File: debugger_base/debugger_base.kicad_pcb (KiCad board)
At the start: 4 copper layers, 58.4 x 38.1 mm, 62 parts, among them SW1 RST_FT, SW2 UART CHx LED enable switch, X1 USB_C_Receptacle_USB2.0_14P, X2 Channel A, X3 Channel B, X4 Channel C, X5 Channel D, Y1 12MHz

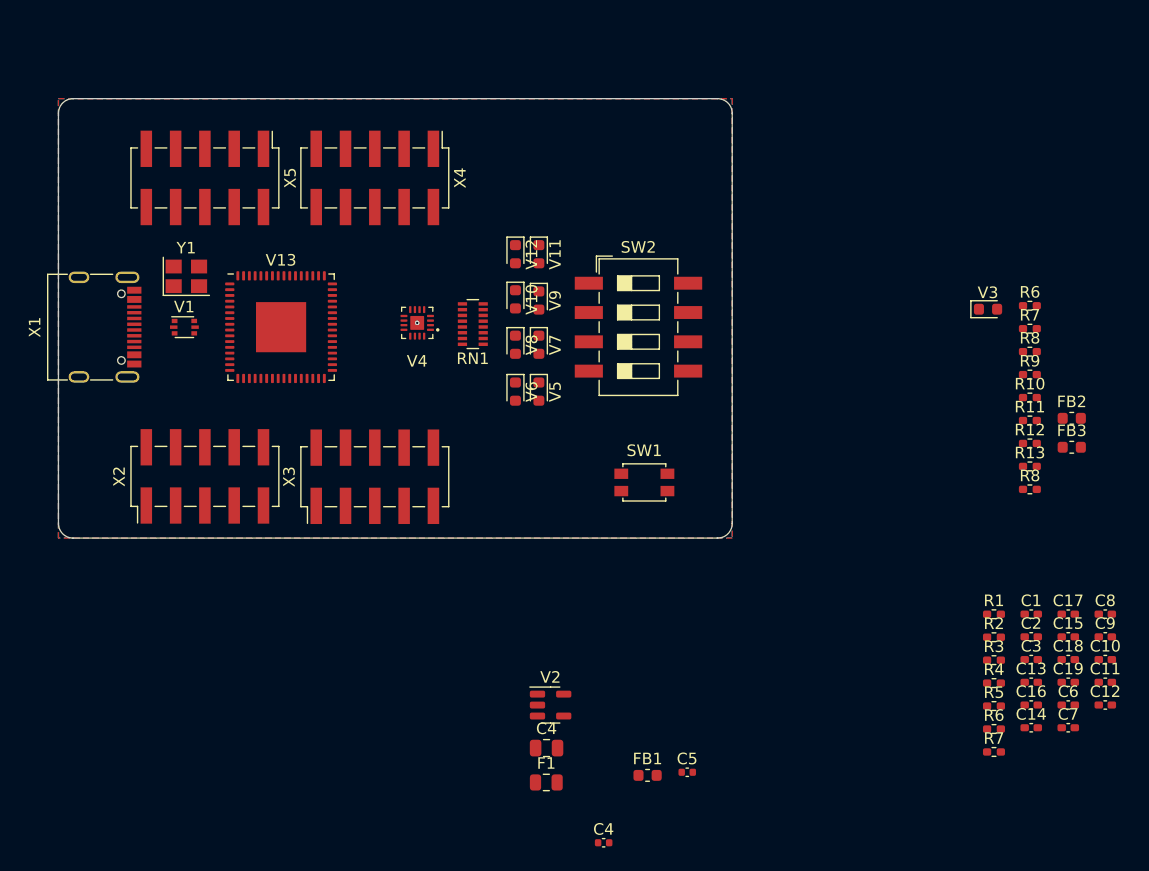
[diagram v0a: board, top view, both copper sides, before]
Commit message: finish base board pcb
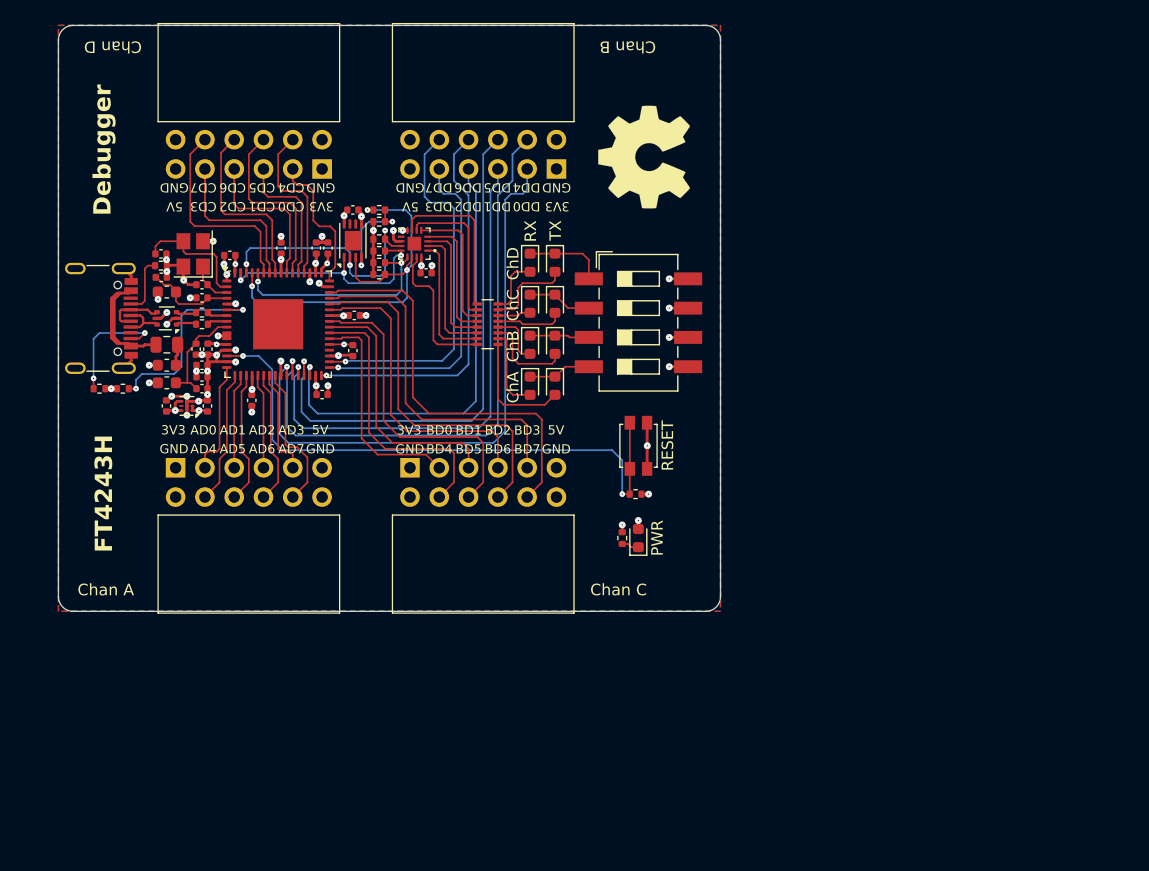
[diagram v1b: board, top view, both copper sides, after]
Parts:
- removed the C4 at (138.8, 119.8)
- removed the C4 at (143.8, 128.0)
- removed the R6 at (180.7, 81.5)
- removed the R6 at (177.6, 118.2)
- removed the R7 at (177.6, 120.1)
- removed the R7 at (180.7, 83.4)
- removed the R8 at (180.7, 85.4)
- removed the R8 at (180.7, 97.4)
- added C20: 100n, Capacitor_SMD:C_0402_1005Metric, F.Cu at (128.4, 78.6)
- added C21: 100n, Capacitor_SMD:C_0402_1005Metric, F.Cu at (122.0, 73.2)
- added C4: 2u2, Capacitor_SMD:C_0402_1005Metric, F.Cu at (109.4, 90.1)
- added R6: 10k, Resistor_SMD:R_0402_1005Metric, F.Cu at (146.6, 97.8)
- added R7: 10k, Resistor_SMD:R_0402_1005Metric, F.Cu at (124.3, 76.7)
- added R8: 10k, Resistor_SMD:R_0402_1005Metric, F.Cu at (124.3, 75.7)
- added REF**: OSHW-Symbol_8.9x8mm_SilkScreen, Symbol:OSHW-Symbol_8.9x8mm_SilkScreen, F.Cu at (147.3, 68.6)
- added V14: RX, LED_SMD:LED_0603_1608Metric, F.Cu at (137.4, 77.7)
- C1: value 2u2 -> 10u; footprint Capacitor_SMD:C_0402_1005Metric_Pad0.74x0.62mm_HandSolder -> Capacitor_SMD:C_0402_1005Metric
- C10, C9: value 4u7 -> 100n; footprint Capacitor_SMD:C_0402_1005Metric_Pad0.74x0.62mm_HandSolder -> Capacitor_SMD:C_0402_1005Metric
- C11, C12, C18, C19, C3: footprint Capacitor_SMD:C_0402_1005Metric_Pad0.74x0.62mm_HandSolder -> Capacitor_SMD:C_0402_1005Metric
- C13, C14: value 100n -> 30p; footprint Capacitor_SMD:C_0402_1005Metric_Pad0.74x0.62mm_HandSolder -> Capacitor_SMD:C_0402_1005Metric
- C15: value 100n -> 3u3; footprint Capacitor_SMD:C_0402_1005Metric_Pad0.74x0.62mm_HandSolder -> Capacitor_SMD:C_0402_1005Metric
- C16, C17: value 100n -> 4u7; footprint Capacitor_SMD:C_0402_1005Metric_Pad0.74x0.62mm_HandSolder -> Capacitor_SMD:C_0402_1005Metric
- C2: value 10n -> 1u; footprint Capacitor_SMD:C_0402_1005Metric_Pad0.74x0.62mm_HandSolder -> Capacitor_SMD:C_0402_1005Metric
- C5: value 1u -> 100n
- C6: value 3u3 -> 100n; footprint Capacitor_SMD:C_0402_1005Metric_Pad0.74x0.62mm_HandSolder -> Capacitor_SMD:C_0402_1005Metric
- C7, C8: value 3p3 -> 100n; footprint Capacitor_SMD:C_0402_1005Metric_Pad0.74x0.62mm_HandSolder -> Capacitor_SMD:C_0402_1005Metric
- F1: value 750mA -> 500mA
- FB2, FB3: value 600R/1A -> FerriteBead_Small
- R1, R2, R3, R4: footprint Resistor_SMD:R_0402_1005Metric_Pad0.72x0.64mm_HandSolder -> Resistor_SMD:R_0402_1005Metric
- R10, R11, R12: value 1k -> 10k; footprint Resistor_SMD:R_0402_1005Metric_Pad0.72x0.64mm_HandSolder -> Resistor_SMD:R_0402_1005Metric
- R13: value 1k -> 2k2; footprint Resistor_SMD:R_0402_1005Metric_Pad0.72x0.64mm_HandSolder -> Resistor_SMD:R_0402_1005Metric
- R5: value 10k -> 1k; footprint Resistor_SMD:R_0402_1005Metric_Pad0.72x0.64mm_HandSolder -> Resistor_SMD:R_0402_1005Metric
- R9: value 1k -> 12k; footprint Resistor_SMD:R_0402_1005Metric_Pad0.72x0.64mm_HandSolder -> Resistor_SMD:R_0402_1005Metric
- SW1: value RST_FT -> RESET
- V13: value FT4232H -> TX; footprint Package_DFN_QFN:QFN-64-1EP_9x9mm_P0.5mm_EP4.35x4.35mm -> LED_SMD:LED_0603_1608Metric
- V2: footprint Package_TO_SOT_SMD:SOT-23-5 -> ft4232_footprints:DFN-6-1EP_1.2x1.2mm_P0.4mm_EP0.3x0.94mm_PullBack
- V4: value 74HC595 -> FT4232HQ; footprint Package_DFN_QFN:Texas_RUM0016A_WQFN-16-1EP_4x4mm_P0.65mm_EP2.6x2.6mm -> Package_DFN_QFN:QFN-64-1EP_9x9mm_P0.5mm_EP4.35x4.35mm
- V5: value TX -> 74HC595; footprint LED_SMD:LED_0603_1608Metric -> ft4232_footprints:74HC595
- V6: value RX -> 93LCxxB; footprint LED_SMD:LED_0603_1608Metric -> Package_DFN_QFN:DFN-8-1EP_3x2mm_P0.5mm_EP1.7x1.4mm
- X1: value USB_C_Receptacle_USB2.0_14P -> USB-C Receptacle; footprint Connector_USB:USB_C_Receptacle_G-Switch_GT-USB-7010ASV -> myLib:USB_C_Receptacle_G-Switch_GT-USB-7010ASV
- X2, X3, X4, X5: footprint Connector_PinHeader_2.54mm:PinHeader_2x05_P2.54mm_Vertical_SMD -> ft4232_footprints:header_female_02x06_613012243121
- moved C11 84.5 mm to (111.4, 77.1)
- moved C13 84.1 mm to (105.4, 77.0), turned to 180 degrees
- moved C17 83.9 mm to (105.4, 79.0), turned to 180 degrees
- moved C19 82.2 mm to (109.0, 80.8)
- moved C12 81.7 mm to (115.8, 76.5), turned to -90 degrees
- moved C14 81.5 mm to (109.0, 79.6)
- moved C7 81.5 mm to (109.5, 85.2), turned to 90 degrees
- moved R2 80.5 mm to (100.1, 88.6)
- moved C18 80.3 mm to (108.5, 85.2), turned to 90 degrees
- moved FB3 79.6 mm to (105.9, 80.3), turned to 180 degrees
- moved R9 78.6 mm to (102.1, 88.6)
- moved FB2 78.5 mm to (105.9, 88.1), turned to 180 degrees
- moved R1 78.3 mm to (105.4, 78.0)
- moved C3 78.1 mm to (105.9, 90.1), turned to 90 degrees
- moved C10 77.2 mm to (118.9, 76.5), turned to -90 degrees
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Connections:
- C1 pad 1: VBUS -> +5V
- C10 pad 2: Net-(V13-VPHY) -> +3V3
- C11 pad 2: Net-(V13-VPLL) -> +1V8
- C12 pad 2: Net-(V13-VPHY) -> +3V3
- C13 pad 2: +1V8 -> Net-(V4-OSCI)
- C14 pad 2: +1V8 -> Net-(V4-OSCO)
- C16 pad 2: +3V3 -> Net-(V4-VPLL)
- C17 pad 2: +3V3 -> Net-(V4-VPHY)
- C18 pad 2: +3V3 -> Net-(V4-VPLL)
- C19 pad 2: +3V3 -> Net-(V4-VPHY)
- C2 pad 1: VBUS -> +5V
- C3 pad 1: +3V3 -> +5V
- C5 pad 1: VBUS -> GND
- C5 pad 2: GND -> +3V3
- C6 pad 2: +1V8 -> +3V3
- C7 pad 2: Net-(V13-OSCI) -> +1V8
- C8 pad 2: Net-(V13-OSCO) -> +3V3
- C9 pad 2: Net-(V13-VPLL) -> +1V8
- FB1 pad 1: VBUS -> +5V
- FB2 pad 1: Net-(V13-VPLL) -> Net-(V4-VPLL)
- FB3 pad 1: Net-(V13-VPHY) -> Net-(V4-VPHY)
- R10 pad 1: unconnected-(R10-Pad1) -> +3V3
- R10 pad 2: unconnected-(R10-Pad2) -> /FT4232H/EE_DATA
- R11 pad 1: unconnected-(R11-Pad1) -> /FT4232H/~{LEDs_ENABLE}
- R11 pad 2: unconnected-(R11-Pad2) -> +3V3
- R12 pad 1: unconnected-(R12-Pad1) -> Net-(V6-DO)
- R12 pad 2: unconnected-(R12-Pad2) -> +3V3
- R13 pad 1: unconnected-(R13-Pad1) -> Net-(V6-DO)
- R13 pad 2: unconnected-(R13-Pad2) -> /FT4232H/EE_DATA
- R3 pad 1: CONN_D- -> Net-(R3-Pad1)
- R3 pad 2: USB_P- -> /FT4232H/USB_P-
- R4 pad 1: CONN_D+ -> Net-(R4-Pad1)
- R4 pad 2: USB_P+ -> /FT4232H/USB_P+
- R9 pad 1: unconnected-(R9-Pad1) -> GND
- R9 pad 2: unconnected-(R9-Pad2) -> Net-(V4-REF)
- SW1 pad 2: ~{RESET} -> /FT4232H/~{RESET}
- SW2 pad 1: CHD_EN -> /LEDs, EEPROM/ChanD_EN
- SW2 pad 2: CHC_EN -> /LEDs, EEPROM/ChanC_EN
- SW2 pad 3: CHB_EN -> /LEDs, EEPROM/ChanB_EN
- SW2 pad 4: CHA_EN -> /LEDs, EEPROM/ChanA_EN
- V1 pad 1: CONN_D+ -> Net-(R4-Pad1)
- V1 pad 3: CONN_D- -> Net-(R3-Pad1)
- V1 pad 4: CONN_D- -> /Power/CONN_D-
- V1 pad 5: VBUS -> +5V
- V1 pad 6: CONN_D+ -> /Power/CONN_D+
- V10 pad 1: CHC_EN -> /LEDs, EEPROM/ChanB_EN
- V10 pad 2: Net-(RN1-R6.1) -> Net-(RN1-R4.1)
- V11 pad 1: CHD_EN -> /LEDs, EEPROM/ChanC_EN
- V11 pad 2: Net-(RN1-R7.1) -> Net-(RN1-R5.1)
- V12 pad 1: CHD_EN -> /LEDs, EEPROM/ChanC_EN
- V12 pad 2: Net-(RN1-R8.1) -> Net-(RN1-R6.1)
- V13 pad 1: GND -> /LEDs, EEPROM/ChanD_EN
- V13 pad 2: Net-(V13-OSCI) -> Net-(RN1-R7.1)
- V2 pad 4: VBUS -> +5V
- V4 pad 1: Net-(RN1-R2.2) -> GND
- V4 pad 10: +3V3 -> GND
- V4 pad 11: EECLK -> GND
- V4 pad 12: EECS -> +1V8
- V4 pad 13: ~{PWREN} -> GND
- V4 pad 14: EEDATA -> /FT4232H/~{RESET}
- V4 pad 15: Net-(RN1-R1.2) -> GND
- V4 pad 16: +3V3 -> /FT4232H/ADBUS0
- V4 pad 2: Net-(RN1-R3.2) -> Net-(V4-OSCI)
- V4 pad 3: Net-(RN1-R4.2) -> Net-(V4-OSCO)
- V4 pad 4: Net-(RN1-R5.2) -> Net-(V4-VPHY)
- V4 pad 5: Net-(RN1-R6.2) -> GND
- V4 pad 6: Net-(RN1-R7.2) -> Net-(V4-REF)
- V4 pad 7: Net-(RN1-R8.2) -> /FT4232H/USB_P-
- V4 pad 8: GND -> /FT4232H/USB_P+
- V4 pad 9: unconnected-(V4-QH'-Pad9) -> Net-(V4-VPLL)
- V5 pad 1: CHA_EN -> Net-(RN1-R2.2)
- V5 pad 2: Net-(RN1-R1.1) -> Net-(RN1-R3.2)
- V6 pad 1: CHA_EN -> /FT4232H/EE_CS
- V6 pad 2: Net-(RN1-R2.1) -> /FT4232H/EE_CLK
- V7 pad 1: CHB_EN -> /LEDs, EEPROM/ChanA_EN
- V7 pad 2: Net-(RN1-R3.1) -> Net-(RN1-R1.1)
- V8 pad 1: CHB_EN -> /LEDs, EEPROM/ChanA_EN
- V8 pad 2: Net-(RN1-R4.1) -> Net-(RN1-R2.1)
- V9 pad 1: CHC_EN -> /LEDs, EEPROM/ChanB_EN
- V9 pad 2: Net-(RN1-R5.1) -> Net-(RN1-R3.1)
- X1 pad A6: CONN_D+ -> /Power/CONN_D+
- X1 pad A7: CONN_D- -> /Power/CONN_D-
- X1 pad B6: CONN_D+ -> /Power/CONN_D+
- X1 pad B7: CONN_D- -> /Power/CONN_D-
- X2 pad 10: /ADBUS7 -> /FT4232H/ADBUS7
- X2 pad 3: /ADBUS0 -> /FT4232H/ADBUS0
- X2 pad 4: /ADBUS4 -> /FT4232H/ADBUS1
- X2 pad 5: /ADBUS1 -> /FT4232H/ADBUS2
- X2 pad 6: /ADBUS5 -> /FT4232H/ADBUS3
- X2 pad 7: /ADBUS2 -> /FT4232H/ADBUS4
- X2 pad 8: /ADBUS6 -> /FT4232H/ADBUS5
- X2 pad 9: /ADBUS3 -> /FT4232H/ADBUS6
- X3 pad 10: /BDBUS7 -> /FT4232H/BDBUS7
- X3 pad 3: /BDBUS0 -> /FT4232H/BDBUS0
- X3 pad 4: /BDBUS4 -> /FT4232H/BDBUS1
- X3 pad 5: /BDBUS1 -> /FT4232H/BDBUS2
- X3 pad 6: /BDBUS5 -> /FT4232H/BDBUS3
- X3 pad 7: /BDBUS2 -> /FT4232H/BDBUS4
- X3 pad 8: /BDBUS6 -> /FT4232H/BDBUS5
- X3 pad 9: /BDBUS3 -> /FT4232H/BDBUS6
- X4 pad 10: /CDBUS7 -> /FT4232H/CDBUS7
- X4 pad 3: /CDBUS0 -> /FT4232H/CDBUS0
- X4 pad 4: /CDBUS4 -> /FT4232H/CDBUS1
- X4 pad 5: /CDBUS1 -> /FT4232H/CDBUS2
- X4 pad 6: /CDBUS5 -> /FT4232H/CDBUS3
- X4 pad 7: /CDBUS2 -> /FT4232H/CDBUS4
- X4 pad 8: /CDBUS6 -> /FT4232H/CDBUS5
- X4 pad 9: /CDBUS3 -> /FT4232H/CDBUS6
- X5 pad 10: /DDBUS7 -> /FT4232H/DDBUS7
- X5 pad 3: /DDBUS0 -> /FT4232H/DDBUS0
- X5 pad 4: /DDBUS4 -> /FT4232H/DDBUS1
- X5 pad 5: /DDBUS1 -> /FT4232H/DDBUS2
- X5 pad 6: /DDBUS5 -> /FT4232H/DDBUS3
- X5 pad 7: /DDBUS2 -> /FT4232H/DDBUS4
- X5 pad 8: /DDBUS6 -> /FT4232H/DDBUS5
- X5 pad 9: /DDBUS3 -> /FT4232H/DDBUS6
- Y1 pad 1: Net-(V13-OSCO) -> Net-(V4-OSCO)
- Y1 pad 2: Net-(V13-OSCI) -> GND
- Y1 pad 3: (no net) -> Net-(V4-OSCI)
- Y1 pad 4: (no net) -> GND
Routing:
- net GND: track 0.00 -> 56.2 mm, vias 0 -> 39
- net /FT4232H/BDBUS1: track 0.00 -> 51.9 mm, vias 0 -> 1
- net /FT4232H/~{RESET}: track 0.00 -> 51.4 mm, vias 0 -> 2
- net /FT4232H/BDBUS0: track 0.00 -> 51.3 mm, vias 0 -> 1
- net +5V: track 0.00 -> 50.3 mm, vias 0 -> 4
- net /FT4232H/BDBUS3: track 0.00 -> 46.1 mm, vias 0 -> 1
- net /FT4232H/BDBUS2: track 0.00 -> 44.9 mm, vias 0 -> 1
- net /FT4232H/BDBUS4: track 0.00 -> 39.7 mm, vias 0 -> 1
- net /FT4232H/EE_DATA: track 0.00 -> 36.0 mm, vias 0 -> 3
- net /FT4232H/CDBUS7: track 0.00 -> 35.3 mm
- net /FT4232H/BDBUS5: track 0.00 -> 33.7 mm, vias 0 -> 1
- net /FT4232H/BDBUS7: track 0.00 -> 31.9 mm, vias 0 -> 1
- net /FT4232H/CDBUS5: track 0.00 -> 31.7 mm
- net /FT4232H/CDBUS6: track 0.00 -> 30.4 mm
- net /FT4232H/BDBUS6: track 0.00 -> 29.5 mm, vias 0 -> 1
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- added copper zone on In2.Cu, net +1V8
- added copper zone on In2.Cu, net +5V
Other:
- board size 58.4 x 38.1 mm -> 57.4 x 50.8 mm
- board text added: "3V3"
- board text added: "5V"
- board text added: "AD0"
- board text added: "AD1"
- board text added: "AD2"
- board text added: "AD3"
- board text added: "AD4"
- board text added: "AD5"
- board text added: "AD6"
- board text added: "AD7"
- board text added: "BD0"
- board text added: "BD1"
- board text added: "BD2"
- board text added: "BD3"
- board text added: "BD4"
- board text added: "BD5"
- board text added: "BD6"
- board text added: "BD7"
- board text added: "CD0"
- board text added: "CD1"
- board text added: "CD2"
- board text added: "CD3"
- board text added: "CD4"
- board text added: "CD5"
- board text added: "CD6"
- board text added: "CD7"
- board text added: "ChA"
- board text added: "ChB"
- board text added: "ChC"
- board text added: "ChD"
- board text added: "Chan A"
- board text added: "Chan B"
- board text added: "Chan C"
- board text added: "Chan D"
- board text added: "DD0"
- board text added: "DD1"
- board text added: "DD2"
- board text added: "DD3"
- board text added: "DD4"
- board text added: "DD5"
- board text added: "DD6"
- board text added: "DD7"
- board text added: "Debugger"
- board text added: "FT4243H"
- board text added: "GND"
- board text added: "RX"
- board text added: "TX"
